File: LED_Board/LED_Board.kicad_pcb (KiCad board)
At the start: 2 copper layers, 34.9 x 34.9 mm, 30 parts, among them J1 Conn_01x03, J10 Conn_01x03, J11 Conn_01x01, J12 Conn_01x01, J13 Conn_01x01, J14 Conn_01x01, J15 Conn_01x01, J16 Conn_01x01, J17 Conn_01x01, J18 Conn_01x01, J19 Conn_01x01, J2 Conn_01x03, J20 Conn_01x01, J3 Conn_01x03, J4 Conn_01x03, J5 Conn_01x03, J6 Conn_01x03, J7 Conn_01x03, J8 Conn_01x03, J9 Conn_01x03

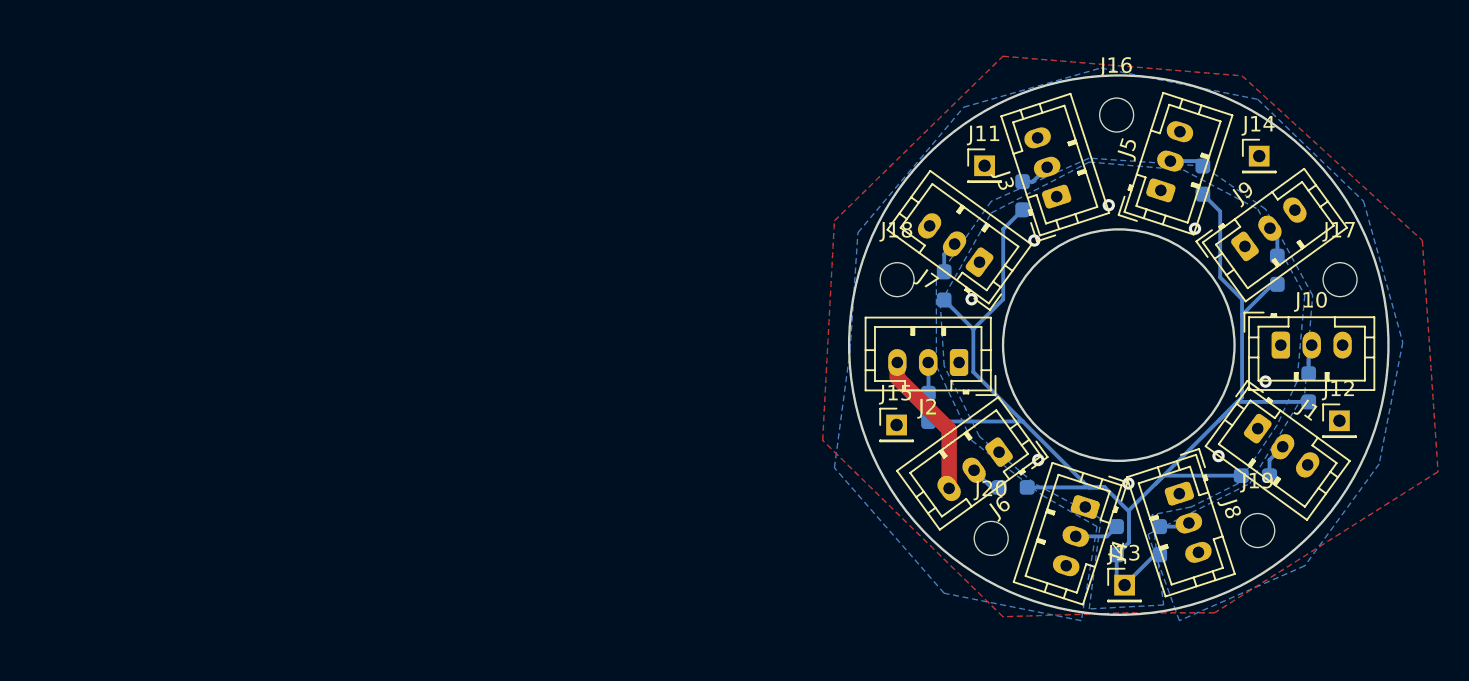
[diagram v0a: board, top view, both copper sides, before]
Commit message: Add files via upload
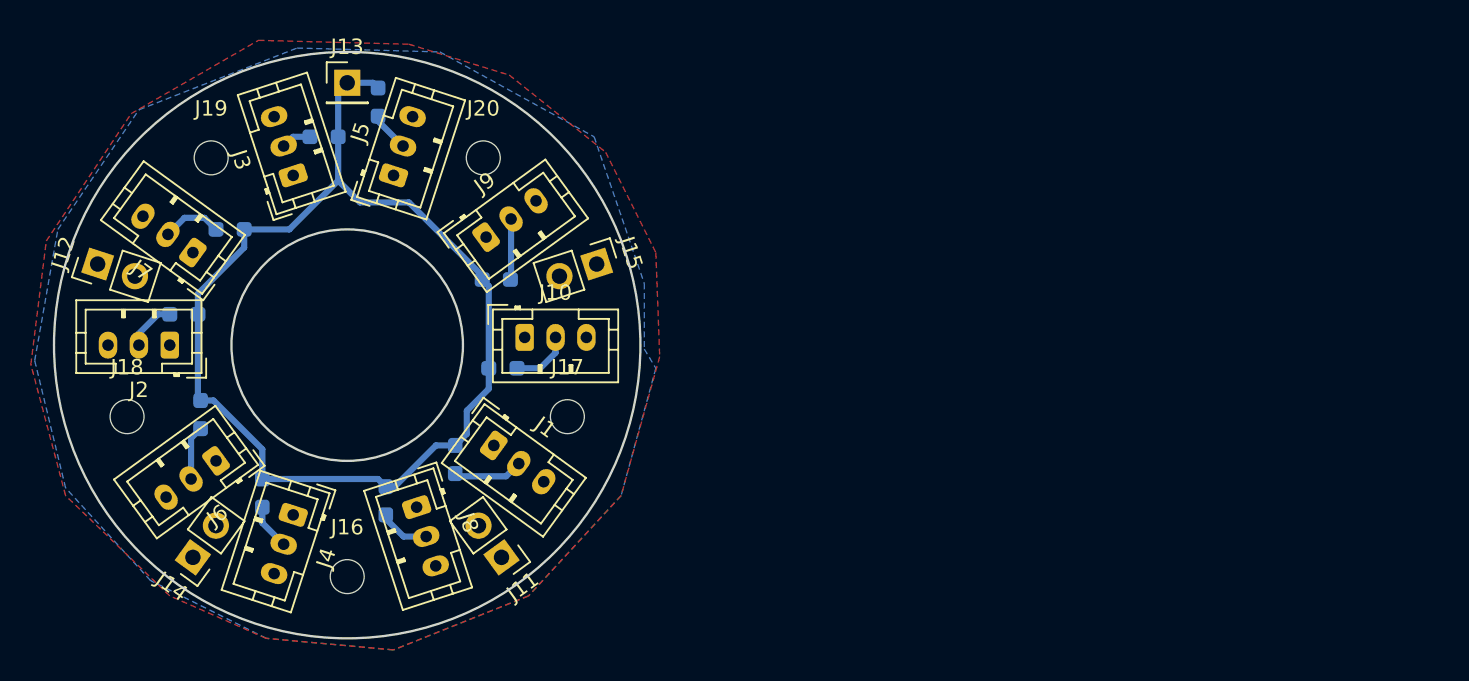
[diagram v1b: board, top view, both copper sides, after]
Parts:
- J11, J12, J14, J15: value Conn_01x01 -> Conn_01x02; footprint Connector_PinHeader_2.00mm:PinHeader_1x01_P2.00mm_Vertical -> Connector_PinHeader_2.54mm:PinHeader_1x02_P2.54mm_Vertical
- J13: footprint Connector_PinHeader_2.00mm:PinHeader_1x01_P2.00mm_Vertical -> Connector_PinHeader_2.54mm:PinHeader_1x01_P2.54mm_Vertical
- moved J12 81.1 mm to (83.8, 94.7), turned to 72 degrees
- moved J14 73.8 mm to (90.0, 113.8), turned to 144 degrees
- moved J19 72.0 mm to (91.2, 87.9)
- moved J13 60.0 mm to (100.0, 83.0)
- moved J16 58.1 mm to (100.0, 115.0)
- moved R4 55.4 mm to (94.5, 109.6), turned to -90 degrees
- moved R5 53.7 mm to (102.0, 84.2), turned to -90 degrees
- moved R6 52.9 mm to (90.5, 104.5), turned to -90 degrees
- moved R10 52.2 mm to (110.1, 101.5), turned to 0 degrees
- moved R1 51.9 mm to (107.0, 107.4), turned to -90 degrees
- moved J4 51.3 mm to (96.5, 111.0)
- moved J2 51.2 mm to (88.5, 100.0)
- moved J7 51.0 mm to (90.0, 94.0)
- moved J17 50.9 mm to (114.3, 104.6)
- moved J6 50.7 mm to (91.5, 107.5)
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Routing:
- net NEO: track 87.7 -> 73.5 mm
- net +5V: track 9.55 -> 0.00 mm
- net Net-(J1-Pad2): track 2.23 -> 4.53 mm
- net Net-(J10-Pad2): track 1.93 -> 3.91 mm
- net Net-(J9-Pad2): track 2.01 -> 3.94 mm
- net Net-(J7-Pad2): track 2.08 -> 3.87 mm
- net Net-(J6-Pad2): track 2.08 -> 3.52 mm
- net Net-(J8-Pad2): track 1.98 -> 3.35 mm
- net Net-(J2-Pad2): track 2.01 -> 3.27 mm
- net GND: vias 8 -> 0
- removed copper zone on B.Cu, net GND
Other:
- board size 34.9 x 34.9 mm -> 38 x 38 mm
- net class Default removed
